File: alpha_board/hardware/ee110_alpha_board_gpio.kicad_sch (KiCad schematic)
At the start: 26 parts, among them J2 4P4C, J6 4P4C, J7 4P4C, J8 4P4C, U2 74LS138, U3 74LVC245, U4 LM9545, U6 MPU-9250

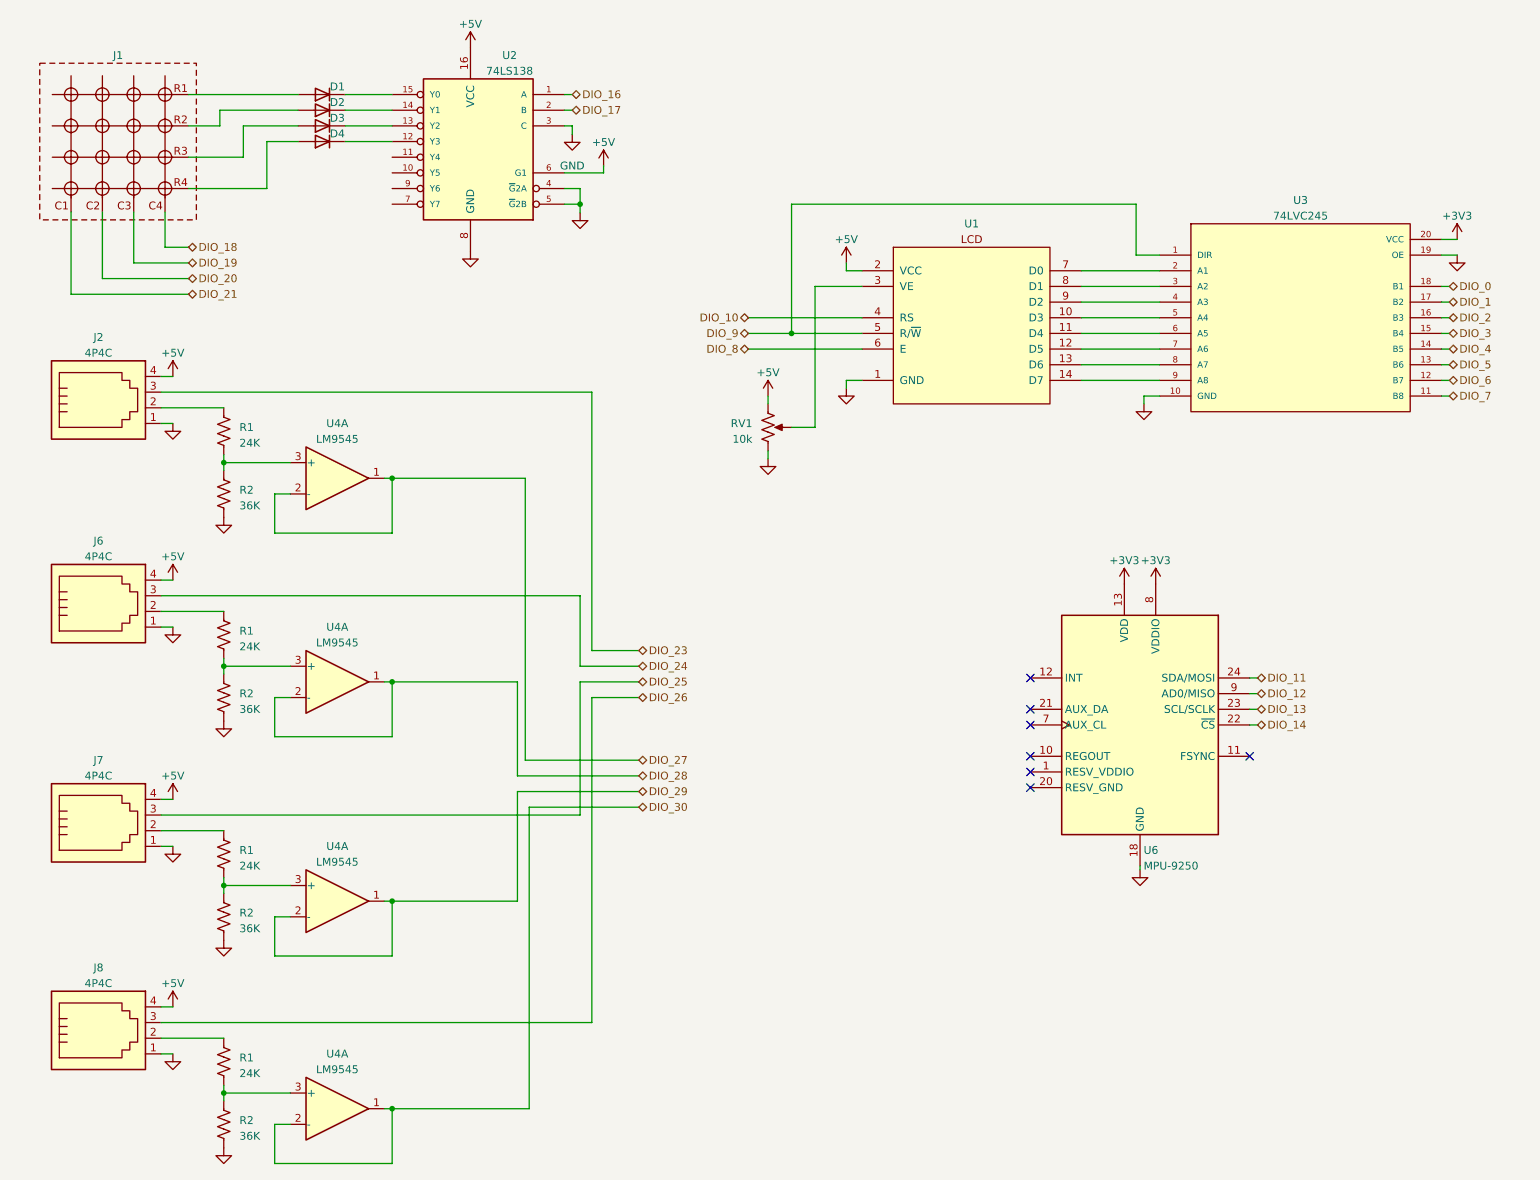
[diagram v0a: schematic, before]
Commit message: biig progress
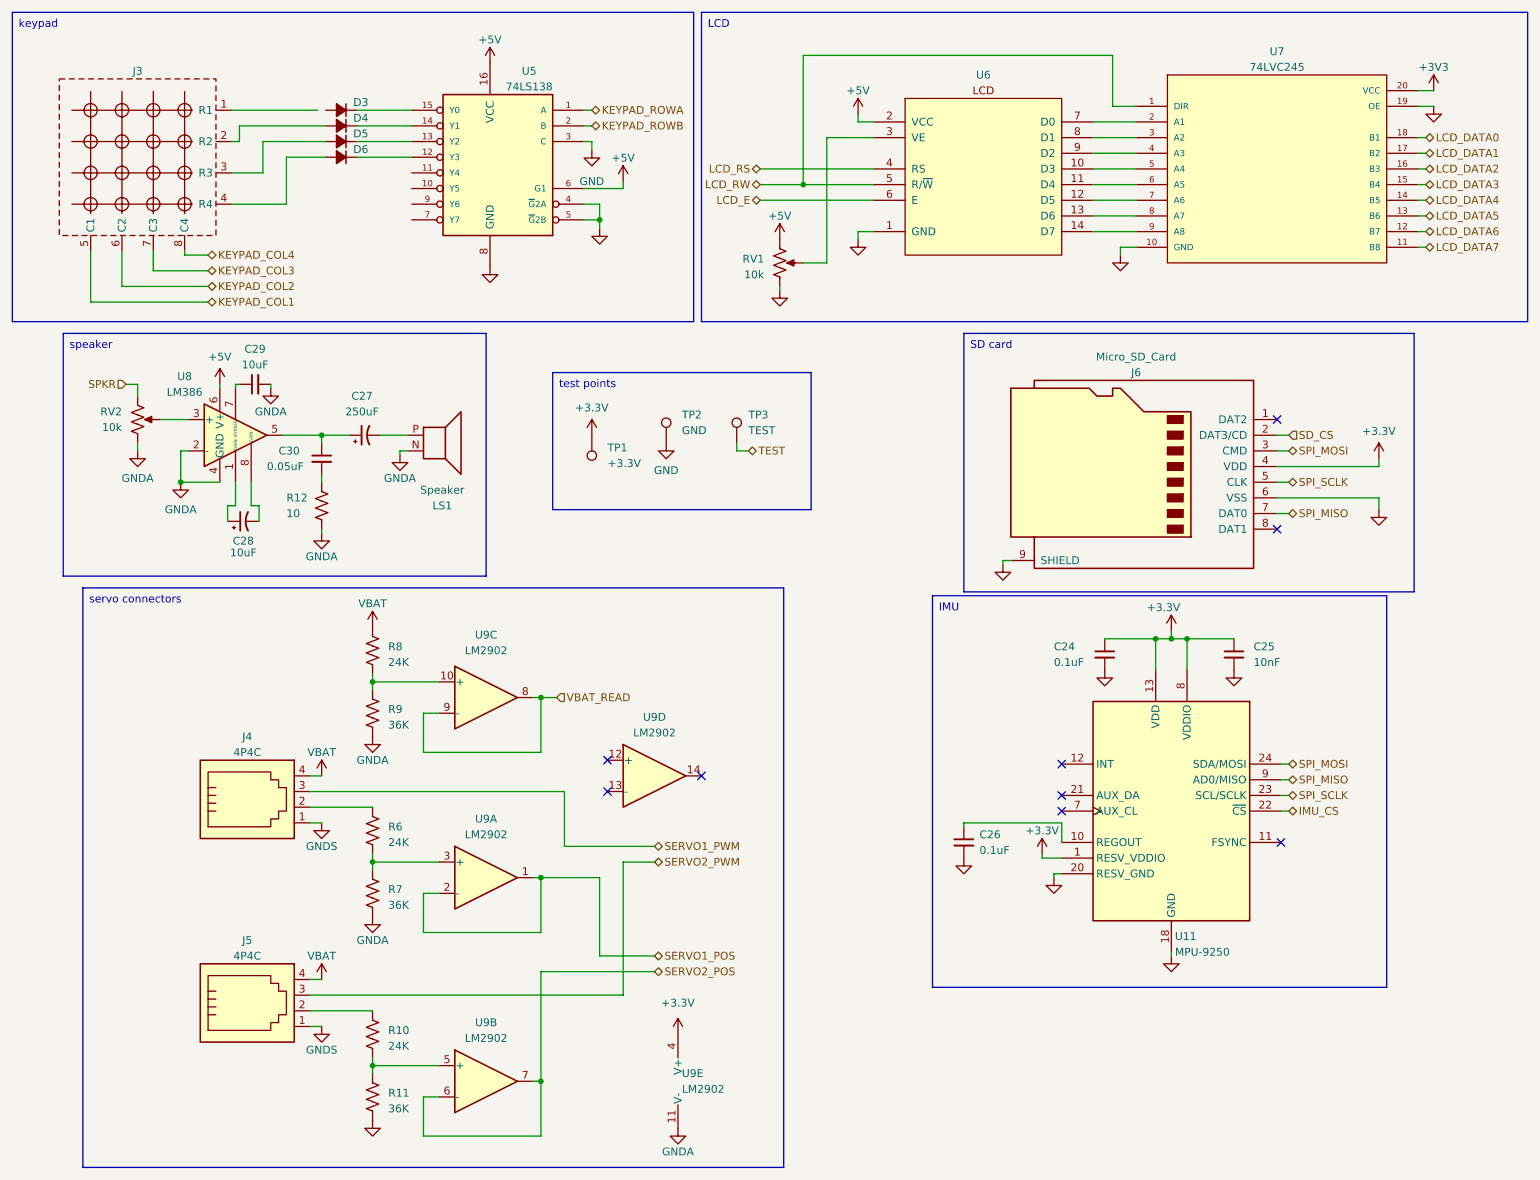
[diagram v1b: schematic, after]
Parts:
- removed D1, D2, D3, D4: 1N4148, Diode_THT:D_DO-35_SOD27_P7.62mm_Horizontal, symbol Diode:1N4148
- removed J7, J8: 4P4C, symbol Connector:4P4C
- removed R1 (x2): 24K, symbol Device:R_US
- removed R2 (x2): 36K, symbol Device:R_US
- removed U4 (x4): LM9545, Package_SO:SOIC-8_3.9x4.9mm_P1.27mm, symbol Amplifier_Operational:TLV9062xD
- added C24, C26: 0.1uF, Capacitor_SMD:C_0603_1608Metric, symbol Device:C_Small
- added C25: 10nF, Capacitor_SMD:C_0603_1608Metric, symbol Device:C_Small
- added C27: 250uF, Capacitor_SMD:C_0603_1608Metric, symbol Device:C_Polarized_Small_US
- added C28: 10uF, Capacitor_SMD:C_0603_1608Metric, symbol Device:C_Polarized_Small_US
- added C29: 10uF, Capacitor_SMD:C_0603_1608Metric, symbol Device:C_Small
- added C30: 0.05uF, Capacitor_SMD:C_0603_1608Metric, symbol Device:C_Small
- added D3, D4, D5, D6: D_Small_Filled, Diode_SMD:D_0603_1608Metric, symbol Device:D_Small_Filled
- added J6: Micro_SD_Card, Connector_Card:microSD_HC_Hirose_DM3D-SF, symbol Connector:Micro_SD_Card
- added LS1: Speaker, My_Footprint:CVS-1508_CUD, symbol Device:Speaker
- added R12: 10, Resistor_SMD:R_0603_1608Metric, symbol Device:R_US
- added R8: 24K, Resistor_SMD:R_0603_1608Metric, symbol Device:R_US
- added R9: 36K, Resistor_SMD:R_0603_1608Metric, symbol Device:R_US
- added RV2: 10k, Potentiometer_THT:Potentiometer_Bourns_3339P_Vertical, symbol Device:R_Potentiometer_US
- added TP1: +3.3V, TestPoint:TestPoint_THTPad_2.0x2.0mm_Drill1.0mm, symbol Connector:TestPoint
- added TP2: GND, TestPoint:TestPoint_THTPad_2.0x2.0mm_Drill1.0mm, symbol Connector:TestPoint
- added TP3: TEST, TestPoint:TestPoint_THTPad_2.0x2.0mm_Drill1.0mm, symbol Connector:TestPoint
- added U8: LM386, Package_DIP:DIP-8-16_W7.62mm, symbol Amplifier_Audio:LM386
- added U9: LM2902, Package_SO:SOIC-14_3.9x8.7mm_P1.27mm, symbol Amplifier_Operational:LM2902
- J3: renamed from J1; footprint (none) -> My_Footprint:4x4_Keypad
- J4: renamed from J2; footprint (none) -> Connector_JST:JST_XH_S4B-XH-A-1_1x04_P2.50mm_Horizontal
- J5: renamed from J6; footprint (none) -> Connector_JST:JST_XH_S4B-XH-A-1_1x04_P2.50mm_Horizontal
- R10, R6: renamed from R1; footprint (none) -> Resistor_SMD:R_0603_1608Metric
- R11, R7: renamed from R2; footprint (none) -> Resistor_SMD:R_0603_1608Metric
- RV1: footprint (none) -> Potentiometer_THT:Potentiometer_Bourns_3339P_Vertical
- U5: renamed from U2; footprint 74LS138:DIL16 -> Package_SO:SOIC-16_3.9x9.9mm_P1.27mm
- U6: renamed from U1; footprint (none) -> Display:LM16255
- U7: renamed from U3; footprint 74LVC245:SOIC-20-W -> Package_SO:SOIC-20W_7.5x15.4mm_P1.27mm
- renumbered U6 to U11
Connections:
- net +3V3: no longer U11.13 (VDD), U11.8 (VDDIO)
- net +5V: now also U8.6 (V+); no longer J4.4, J5.4
- net GND: now also U11.20 (RESV_GND), C24.2, C25.2, C26.2, J6.6 (VSS), J6.9 (SHIELD), TP2.1; no longer J4.1, J5.1, R11.2, R7.2
- net +3.3V: now reaches U11.1 (RESV_VDDIO)
- net +3.3V: now also U11.13 (VDD), U11.8 (VDDIO), C24.1, C25.1, J6.4 (VDD), TP1.1, U9.4 (V+)
- net at U11.10 (REGOUT): now also C26.1
- net at U5.12 (Y3): now also D6.1 (K)
- net at R6.2, R7.1: now also U9.3 (+)
- net at U5.15 (Y0): now also D3.1 (K)
- net at R10.2, R11.1: now also U9.5 (+)
- net at U5.13 (Y2): now also D5.1 (K)
- net at U5.14 (Y1): now also D4.1 (K)
- net DIO_0 renamed LCD_DATA0
- net DIO_1 renamed LCD_DATA1
- net DIO_10 renamed LCD_RS
- net DIO_11 renamed SPI_MOSI
- net SPI_MOSI: now also J6.3 (CMD)
- net DIO_12 renamed SPI_MISO
- net SPI_MISO: now also J6.7 (DAT0)
- net DIO_13 renamed SPI_SCLK
- net SPI_SCLK: now also J6.5 (CLK)
- net DIO_14 renamed IMU_CS
- net DIO_16 renamed KEYPAD_ROWA
- net DIO_17 renamed KEYPAD_ROWB
- removed net DIO_18: J3.
- removed net DIO_19: J3.
- net DIO_2 renamed LCD_DATA2
- removed net DIO_20: J3.
- removed net DIO_21: J3.
- net DIO_23 renamed SERVO1_PWM
- net DIO_24 renamed SERVO2_PWM
- net DIO_3 renamed LCD_DATA3
- net DIO_4 renamed LCD_DATA4
- net DIO_5 renamed LCD_DATA5
- net DIO_6 renamed LCD_DATA6
- net DIO_7 renamed LCD_DATA7
- net DIO_8 renamed LCD_E
- net DIO_9 renamed LCD_RW
- new net: R8.2, R9.1, U9.10 (+)
- new net: D5.2 (A), J3.3 (R3)
- new net: D6.2 (A), J3.4 (R4)
- new net: RV2.2, U8.3 (+)
- new net: D4.2 (A), J3.2 (R2)
- new net: C27.1, C30.1, U8.5
- new net: C30.2, R12.1
- new net: C27.2, LS1.P (1)
- new net: C28.1, U8.1 (GAIN)
- new net: C29.1, U8.7 (BYPASS)
- new net: C28.2, U8.8 (GAIN)
- new net +5VD: J4.4, J5.4, R8.1
- new net GNDA: C29.2, LS1.N (2), R11.2, R12.2, R7.2, R9.2, RV2.3, U8.2 (-), U8.4 (GND), U9.11 (V-)
- new net GNDS: J4.1, J5.1
- new net KEYPAD_COL1: J3.5 (C1)
- new net KEYPAD_COL2: J3.6 (C2)
- new net KEYPAD_COL3: J3.7 (C3)
- new net KEYPAD_COL4: J3.8 (C4)
- new net SD_CS: J6.2 (DAT3/CD)
- new net SERVO1_POS: U9.1, U9.2 (-)
- new net SERVO2_POS: U9.6 (-), U9.7
- new net SPKR: RV2.1
- new net TEST: TP3.1
- new net VBAT_READ: U9.8, U9.9 (-)
- no-connect marks 7 -> 9
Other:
- moved on the sheet: J4, J5, R10, R11, R6, R7, RV1, U11, U5, U6, U7
